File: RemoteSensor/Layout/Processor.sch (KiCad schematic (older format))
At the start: 21 parts, among them J3 LCD_HEADER, Q3 2N7002, SW2 SW_Push, U7 ESP-12F, U8 LM50CIM3, U9 MCP23008-E_P

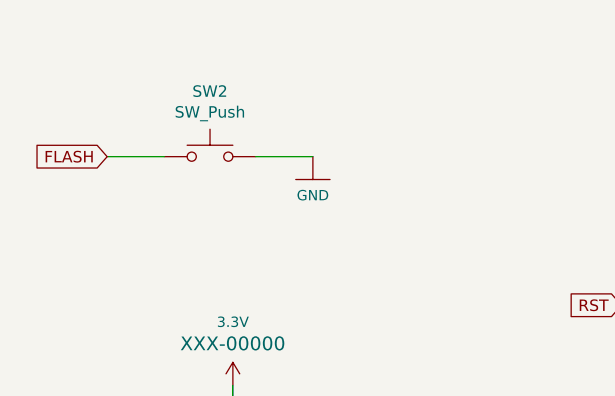
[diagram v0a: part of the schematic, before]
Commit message: Update outputs
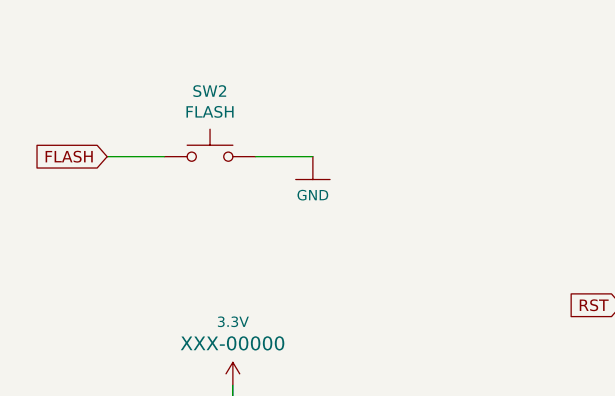
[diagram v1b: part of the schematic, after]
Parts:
- SW2: value SW_Push -> FLASH
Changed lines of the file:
@@
 P 2100 1300
 F 0 "SW2" H 2100 1585 50  0000 C CNN
-F 1 "SW_Push" H 2100 1494 50  0000 C CNN
+F 1 "FLASH" H 2100 1494 50  0000 C CNN
 F 2 "Button_Switch_SMD:SW_SPST_TL3342" H 2100 1500 50  0001 C CNN
 F 3 "~" H 2100 1500 50  0001 C CNN
